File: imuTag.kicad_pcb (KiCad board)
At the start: 4 copper layers, 41.3 x 40 mm, 47 parts, among them J1 Conn_02x05_Odd_Even, J2 Conn_01x05_Socket, J3 Conn_01x02_Pin, Q1 DMG2305UX-13, U1 E73-2G4M08S1C, U2 ME6211C30M5G-N, U3 GD25Q64ESIG, U4 LSM6DSV16XTR, U5 LIS2MDLTR, Y2 Crystal

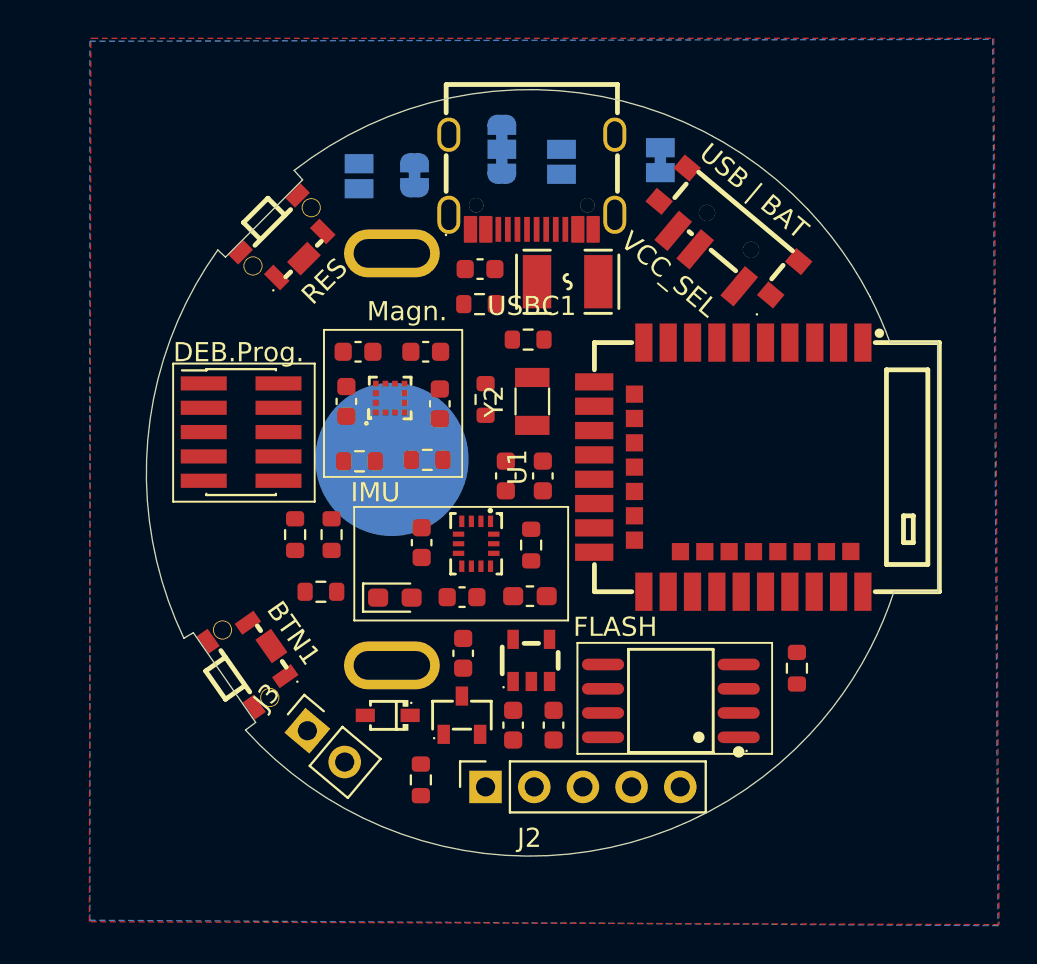
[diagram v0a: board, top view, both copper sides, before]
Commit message: Save current routing work
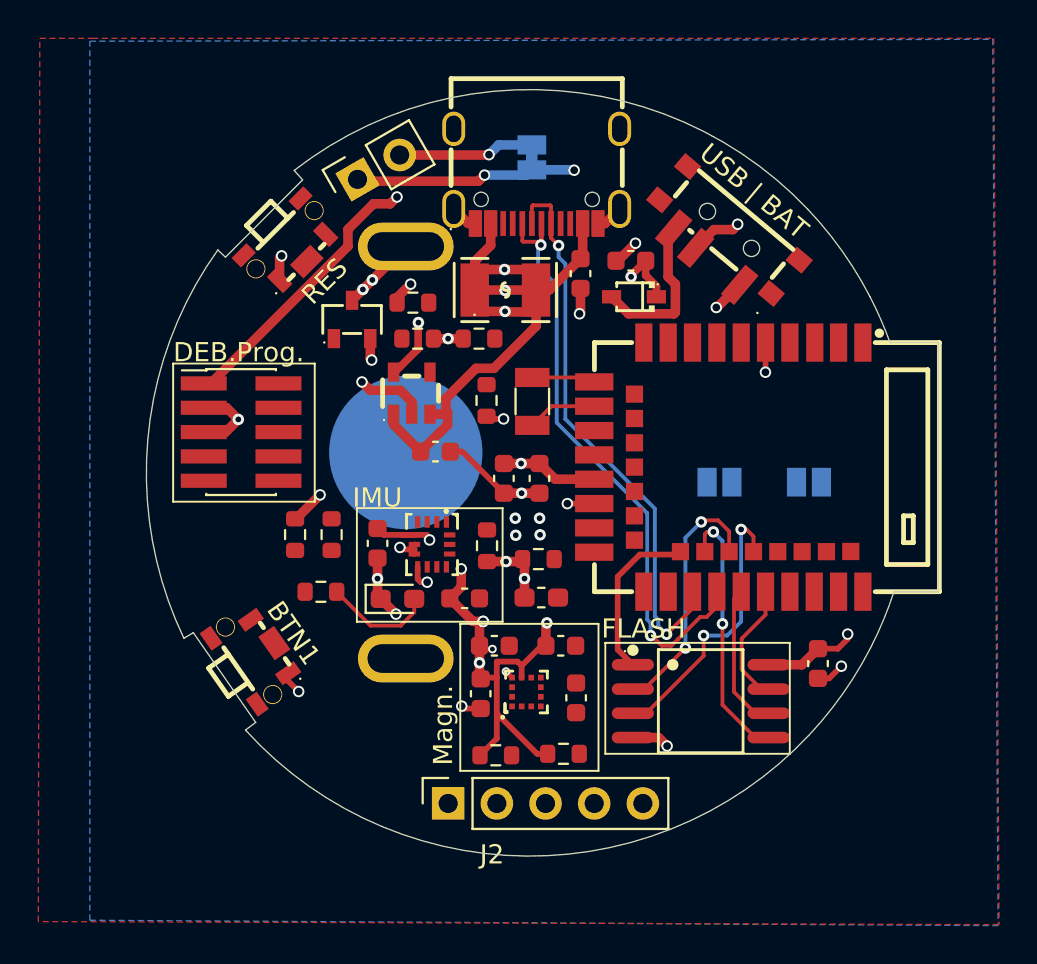
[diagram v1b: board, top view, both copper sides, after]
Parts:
- removed JP6: SolderJumper_3_Bridged123, Jumper:SolderJumper-3_P1.3mm_Bridged123_RoundedPad1.0x1.5mm
- removed JP9: SolderJumper_2_Bridged, Jumper:SolderJumper-2_P1.3mm_Bridged_RoundedPad1.0x1.5mm
- moved J3 28.9 mm to (160.5, 84.8), turned to 120 degrees
- moved D3 25.3 mm to (174.9, 90.9)
- moved JP1 24.7 mm to (179.4, 100.6), turned to 180 degrees
- moved R6 23.0 mm to (163.6, 93.1), turned to 180 degrees
- moved C3 22.3 mm to (174.8, 89.1), turned to 180 degrees
- moved Q1 21.4 mm to (160.2, 92.1)
- moved JP7 21.1 mm to (184.1, 100.6), turned to 180 degrees
- moved C16 16.9 mm to (171.9, 111.9)
- moved C17 16.9 mm to (167.6, 109.1)
- moved R16 16.9 mm to (167.7, 114.9)
- moved R18 16.9 mm to (171.2, 114.8)
- moved U5 16.9 mm to (169.3, 111.6)
- moved C21 16.9 mm to (171.1, 109.1)
- moved C19 16.8 mm to (166.9, 111.6)
- moved U2 15.3 mm to (163.3, 96.0)
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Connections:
- net Net-(J3-Pin_1) renamed /VCC_1
- BAT1 pad 1: Net-(Q1-D) -> /VBAT
- Q1 pad 2: /VBAT -> /VBAT1
- Q1 pad 3: Net-(Q1-D) -> /VBAT
- R15 pad 2: Net-(JP9-A) -> Net-(JP7-B)
- R16 pad 1: Net-(JP6-B) -> VCC
- R18 pad 1: Net-(JP6-A) -> VCC
- U1 pad 16: /LIS2MDL_INT -> /LSM6DSV16_INT2
- U1 pad 17: unconnected-(U1-P1.09-Pad17) -> /LSM6DSV16_INT2
- U1 pad 38: /LSM6DSV16_INT2 -> /LIS2MDL_INT
- VCCSEL1 pad 1: /VBAT -> /VBAT1
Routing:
- net VCC: track 0.00 -> 70.7 mm, vias 0 -> 20
- net /+5V_USB: track 0.00 -> 36.8 mm, vias 0 -> 3
- net GND: track 0.00 -> 36.4 mm, vias 0 -> 17
- net /USB_D+: track 0.00 -> 32.2 mm, vias 0 -> 2
- net /USB_D-: track 0.00 -> 29.8 mm, vias 0 -> 2
- net /VCC_1: track 0.00 -> 24.9 mm, vias 0 -> 3
- net /VBAT1: track 0.00 -> 22.0 mm, vias 0 -> 2
- net Net-(D3-K): track 0.00 -> 18.6 mm, vias 0 -> 2
- net /QSPI_IO2: track 0.00 -> 14.6 mm, vias 0 -> 2
- net /QSPI_IO0: track 0.00 -> 13.7 mm, vias 0 -> 2
- net /QSPI_IO1: track 0.00 -> 13.3 mm, vias 0 -> 2
- net /USB_3V0: track 0.00 -> 9.07 mm
- net /QSPI_CS: track 0.00 -> 8.74 mm
- net /QSPI_CLK: track 0.00 -> 7.65 mm
- net /QSPI_IO3: track 0.00 -> 6.40 mm
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- added copper zone on F.Cu, net GND
- added copper zone on In1.Cu, net GND
- removed copper zone on In1.Cu, net (none)
- removed copper zone on F.Cu, net /VBAT
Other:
- board text removed: "VCC_SEL"
